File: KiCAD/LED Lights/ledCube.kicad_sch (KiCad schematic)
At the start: 14 parts, among them P1 CONN_01X03, P2 CONN_01X02, P3 CONN_01X02, P4 CONN_01X02, P5 CONN_01X02, U1 AL8805W5

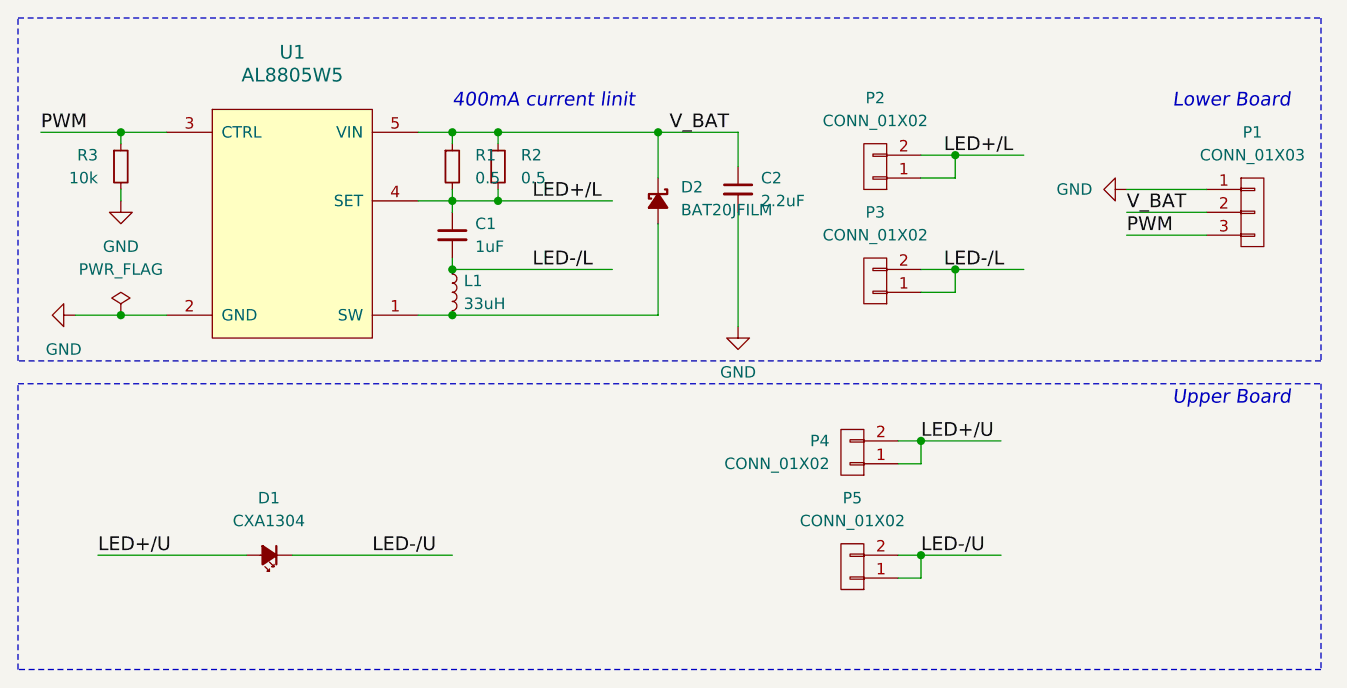
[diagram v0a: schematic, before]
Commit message: clean up
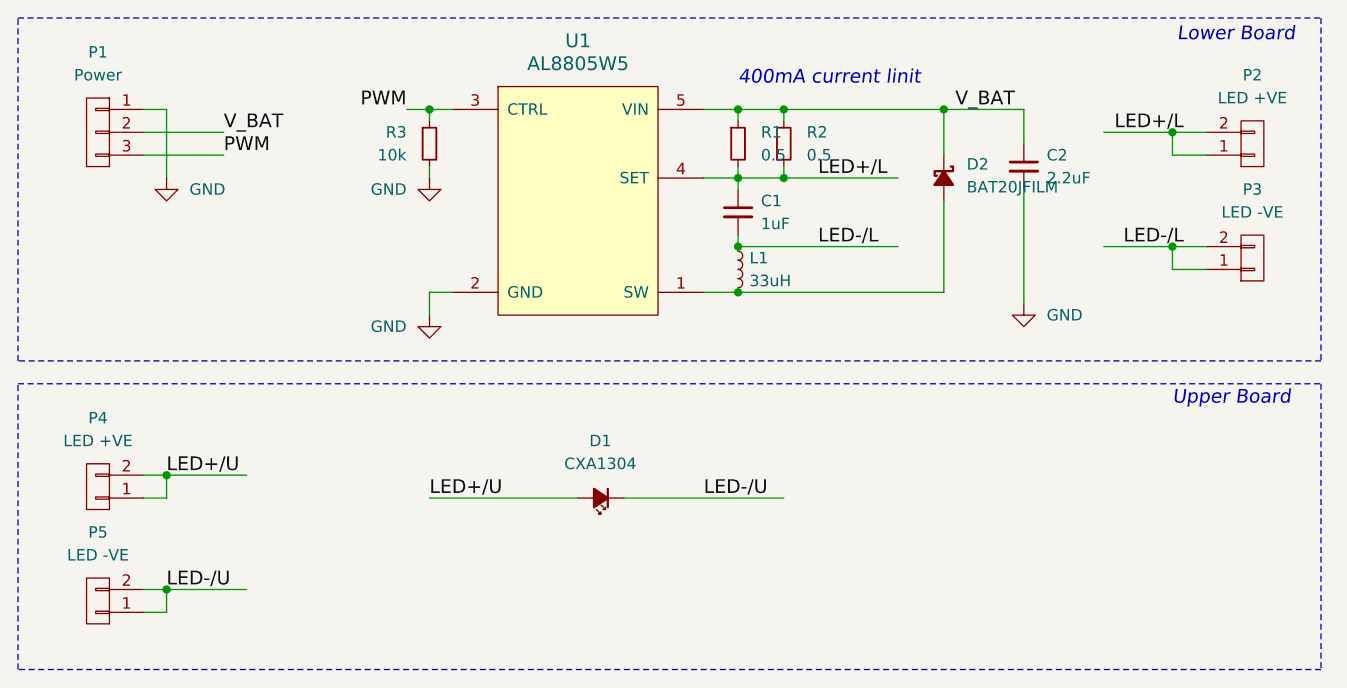
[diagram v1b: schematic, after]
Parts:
- P1: value CONN_01X03 -> Power
- P2, P4: value CONN_01X02 -> LED +VE
- P3, P5: value CONN_01X02 -> LED -VE
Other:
- moved on the sheet: C1, C2, D1, D2, L1, P1, P2, P3, P4, P5, R1, R2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
